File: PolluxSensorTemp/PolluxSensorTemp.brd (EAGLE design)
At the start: 22.5 x 19 mm, 4 parts

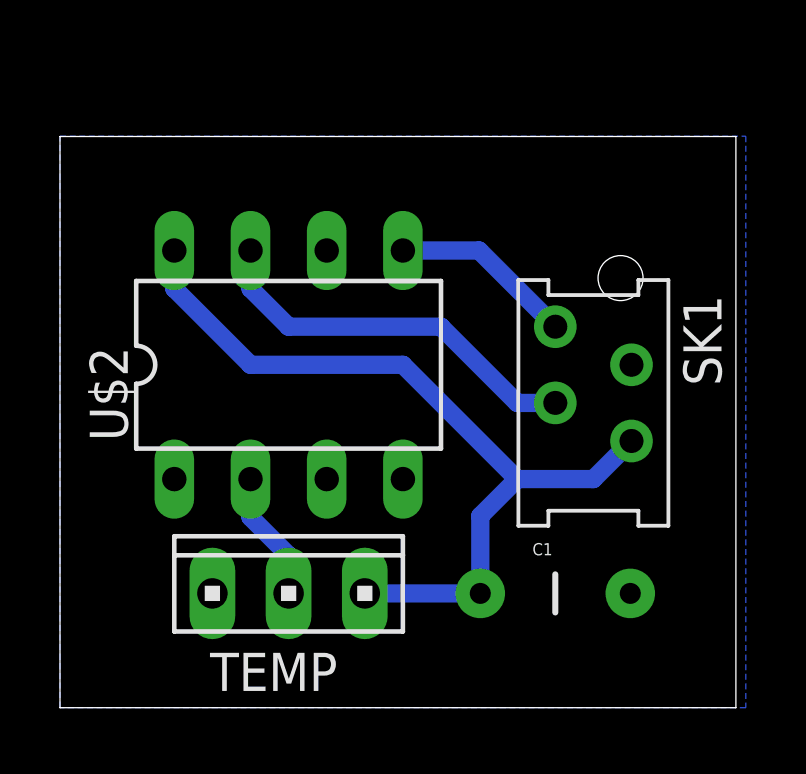
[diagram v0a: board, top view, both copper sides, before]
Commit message: improve sensor board
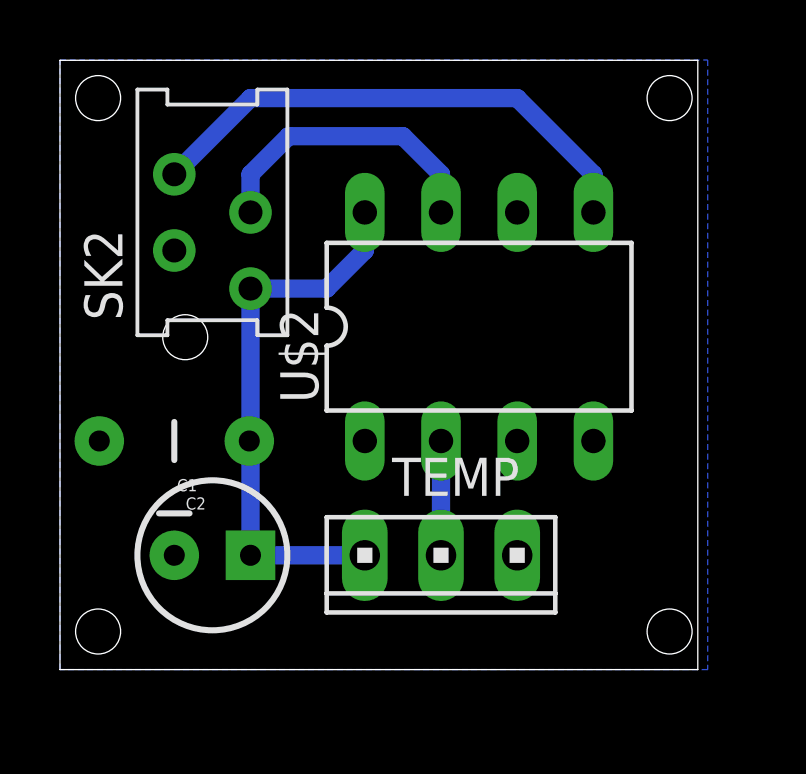
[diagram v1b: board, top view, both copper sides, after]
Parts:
- removed SK1: (no value), jt-con-micromatch:AMP-215079-8
- added C2: 1 uF, SparkFun:CPOL-RADIAL-10UF-25V
- added SK2: (no value), jt-con-micromatch:AMP-215079-8
- C1: value (none) -> 10 pF
- moved C1 13.7 mm to (15.2, 16.5), turned to 180 degrees
- moved U$2 6.48 mm to (25.4, 20.3)
- moved TEMP 5.24 mm to (24.1, 12.7), turned to 180 degrees
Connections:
- removed net N$2: SK1.1, U$2.5
- new net SDA: SK2.4, U$2.5
- net 5V: now also C2.1, SK2.1; no longer SK1.4
- net GND: now also C2.2, SK2.2; no longer SK1.2
- net N$1: now also SK2.3; no longer SK1.3
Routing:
- net SDA: track 0.00 -> 17.3 mm
- net 5V: track 27.8 -> 18.3 mm
- net N$2: track 6.13 -> 0.00 mm
- net N$1: track 13.0 -> 9.94 mm
- net READ: track 4.34 -> 3.81 mm
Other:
- board size 22.5 x 19 mm -> 21.3 x 20.3 mm
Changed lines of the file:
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@@
 <layer number="43" name="vRestrict" color="2" fill="10" visible="yes" active="yes"/>
 <layer number="44" name="Drills" color="7" fill="1" visible="no" active="yes"/>
-<layer number="45" name="Holes" color="7" fill="1" visible="no" active="yes"/>
+<layer number="45" name="Holes" color="7" fill="1" visible="yes" active="yes"/>
 <layer number="46" name="Milling" color="3" fill="1" visible="no" active="yes"/>
 <layer number="47" name="Measures" color="7" fill="1" visible="no" active="yes"/>
@@
 <board>
 <plain>
-<wire x1="11.43" y1="7.62" x2="33.96" y2="7.62" width="0" layer="20"/>
-<wire x1="33.96" y1="7.62" x2="33.96" y2="26.66" width="0" layer="20"/>
-<wire x1="33.96" y1="26.66" x2="11.43" y2="26.66" width="0" layer="20"/>
-<wire x1="11.43" y1="26.66" x2="11.43" y2="7.62" width="0" layer="20"/>
+<wire x1="11.43" y1="8.89" x2="32.69" y2="8.89" width="0" layer="20"/>
+<wire x1="32.69" y1="8.89" x2="32.69" y2="29.2" width="0" layer="20"/>
+<wire x1="32.69" y1="29.2" x2="11.43" y2="29.2" width="0" layer="20"/>
+<wire x1="11.43" y1="29.2" x2="11.43" y2="8.89" width="0" layer="20"/>
+<hole x="12.7" y="27.94" drill="1.5"/>
+<hole x="12.7" y="10.16" drill="1.5"/>
+<hole x="31.75" y="10.16" drill="1.5"/>
+<hole x="31.75" y="27.94" drill="1.5"/>
 </plain>
 <attributes>
@@
 </autorouter>
 <elements>
-<element name="SK1" library="jt-con-micromatch" package="AMP-215079-8" value="" x="29.21" y="20.32" rot="R270"/>
-<element name="U$2" library="avr-7" package="DIL08" value="TINY25/45/85-20PU" x="19.05" y="19.05"/>
-<element name="TEMP" library="con-amp" package="10X03MTA" value="" x="19.05" y="11.43"/>
-<element name="C1" library="SparkFun" package="CAP-PTH-5MM" value="" x="27.94" y="11.43"/>
+<element name="U$2" library="avr-7" package="DIL08" value="TINY25/45/85-20PU" x="25.4" y="20.32"/>
+<element name="TEMP" library="con-amp" package="10X03MTA" value="" x="24.13" y="12.7" rot="R180"/>
+<element name="C1" library="SparkFun" package="CAP-PTH-5MM" value="10 pF" x="15.24" y="16.51" rot="R180"/>
+<element name="SK2" library="jt-con-micromatch" package="AMP-215079-8" value="" x="16.51" y="21.59" rot="R90"/>
+<element name="C2" library="SparkFun" package="CPOL-RADIAL-10UF-25V" value="1 uF" x="16.51" y="12.7"/>
 </elements>
 <signals>
-<signal name="N$2">
-<contactref element="SK1" pad="1"/>
-<contactref element="U$2" pad="5"/>
-<wire x1="22.86" y1="22.86" x2="25.4" y2="22.86" width="0.6096" layer="16"/>
-<wire x1="25.4" y1="22.86" x2="27.94" y2="20.32" width="0.6096" layer="16"/>
-</signal>
 <signal name="5V">
-<contactref element="SK1" pad="4"/>
 <contactref element="U$2" pad="8"/>
 <contactref element="C1" pad="1"/>
 <contactref element="TEMP" pad="1"/>
-<wire x1="21.59" y1="11.43" x2="25.44" y2="11.43" width="0.6096" layer="16"/>
-<wire x1="15.24" y1="22.86" x2="15.24" y2="21.59" width="0.6096" layer="16"/>
-<wire x1="15.24" y1="21.59" x2="17.78" y2="19.05" width="0.6096" layer="16"/>
-<wire x1="17.78" y1="19.05" x2="22.86" y2="19.05" width="0.6096" layer="16"/>
-<wire x1="22.86" y1="19.05" x2="26.67" y2="15.24" width="0.6096" layer="16"/>
-<wire x1="26.67" y1="15.24" x2="29.21" y2="15.24" width="0.6096" layer="16"/>
-<wire x1="29.21" y1="15.24" x2="30.48" y2="16.51" width="0.6096" layer="16"/>
-<wire x1="25.44" y1="11.43" x2="25.44" y2="14.01" width="0.6096" layer="16"/>
-<wire x1="25.44" y1="14.01" x2="26.67" y2="15.24" width="0.6096" layer="16"/>
+<contactref element="SK2" pad="1"/>
+<contactref element="C2" pad="1"/>
+<wire x1="17.78" y1="21.59" x2="20.32" y2="21.59" width="0.6096" layer="16"/>
+<wire x1="20.32" y1="21.59" x2="21.59" y2="22.86" width="0.6096" layer="16"/>
+<wire x1="21.59" y1="22.86" x2="21.59" y2="24.13" width="0.6096" layer="16"/>
+<wire x1="17.78" y1="21.59" x2="17.78" y2="16.51" width="0.6096" layer="16"/>
+<wire x1="17.78" y1="16.51" x2="17.74" y2="16.51" width="0.6096" layer="16"/>
+<wire x1="17.78" y1="16.51" x2="17.78" y2="12.7" width="0.6096" layer="16"/>
+<wire x1="17.78" y1="12.7" x2="21.59" y2="12.7" width="0.6096" layer="16"/>
 </signal>
 <signal name="GND">
 <contactref element="U$2" pad="4"/>
-<contactref element="SK1" pad="2"/>
 <polygon width="0.4064" layer="16" orphans="yes">
-<vertex x="11.43" y="26.67"/>
-<vertex x="34.29" y="26.67"/>
-<vertex x="34.29" y="7.62"/>
-<vertex x="11.43" y="7.62"/>
+<vertex x="11.43" y="29.21"/>
+<vertex x="33.02" y="29.21"/>
+<vertex x="33.02" y="8.89"/>
+<vertex x="11.43" y="8.89"/>
 </polygon>
 <contactref element="TEMP" pad="3"/>
 <contactref element="C1" pad="2"/>
+<contactref element="C2" pad="2"/>
+<contactref element="SK2" pad="2"/>
 </signal>
 <signal name="N$1">
 <contactref element="U$2" pad="7"/>
-<contactref element="SK1" pad="3"/>
-<wire x1="17.78" y1="22.86" x2="17.78" y2="21.59" width="0.6096" layer="16"/>
-<wire x1="17.78" y1="21.59" x2="19.05" y2="20.32" width="0.6096" layer="16"/>
-<wire x1="19.05" y1="20.32" x2="24.13" y2="20.32" width="0.6096" layer="16"/>
-<wire x1="24.13" y1="20.32" x2="26.67" y2="17.78" width="0.6096" layer="16"/>
-<wire x1="26.67" y1="17.78" x2="27.94" y2="17.78" width="0.6096" layer="16"/>
+<contactref element="SK2" pad="3"/>
+<wire x1="17.78" y1="24.13" x2="17.78" y2="25.4" width="0.6096" layer="16"/>
+<wire x1="17.78" y1="25.4" x2="19.05" y2="26.67" width="0.6096" layer="16"/>
+<wire x1="19.05" y1="26.67" x2="22.86" y2="26.67" width="0.6096" layer="16"/>
+<wire x1="22.86" y1="26.67" x2="24.13" y2="25.4" width="0.6096" layer="16"/>
+<wire x1="24.13" y1="25.4" x2="24.13" y2="24.13" width="0.6096" layer="16"/>
 </signal>
 <signal name="READ">
 <contactref element="U$2" pad="2"/>
 <contactref element="TEMP" pad="2"/>
-<wire x1="17.78" y1="15.24" x2="17.78" y2="13.97" width="0.6096" layer="16"/>
-<wire x1="17.78" y1="13.97" x2="19.05" y2="12.7" width="0.6096" layer="16"/>
-<wire x1="19.05" y1="12.7" x2="19.05" y2="11.43" width="0.6096" layer="16"/>
+<wire x1="24.13" y1="12.7" x2="24.13" y2="16.51" width="0.6096" layer="16"/>
+</signal>
+<signal name="SDA">
+<contactref element="U$2" pad="5"/>
+<contactref element="SK2" pad="4"/>
+<wire x1="15.24" y1="25.4" x2="17.78" y2="27.94" width="0.6096" layer="16"/>
+<wire x1="17.78" y1="27.94" x2="26.67" y2="27.94" width="0.6096" layer="16"/>
+<wire x1="26.67" y1="27.94" x2="29.21" y2="25.4" width="0.6096" layer="16"/>
+<wire x1="29.21" y1="25.4" x2="29.21" y2="24.13" width="0.6096" layer="16"/>
 </signal>
 </signals>
